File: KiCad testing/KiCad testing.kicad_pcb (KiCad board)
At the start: 2 copper layers, 101.6 x 127 mm, 37 parts, among them J1 USB_A, Q1 IRF540N, Q2 IRF540N, Q3 IRF540N, Q4 IRF540N, U1 IR2213, U4 IR2213

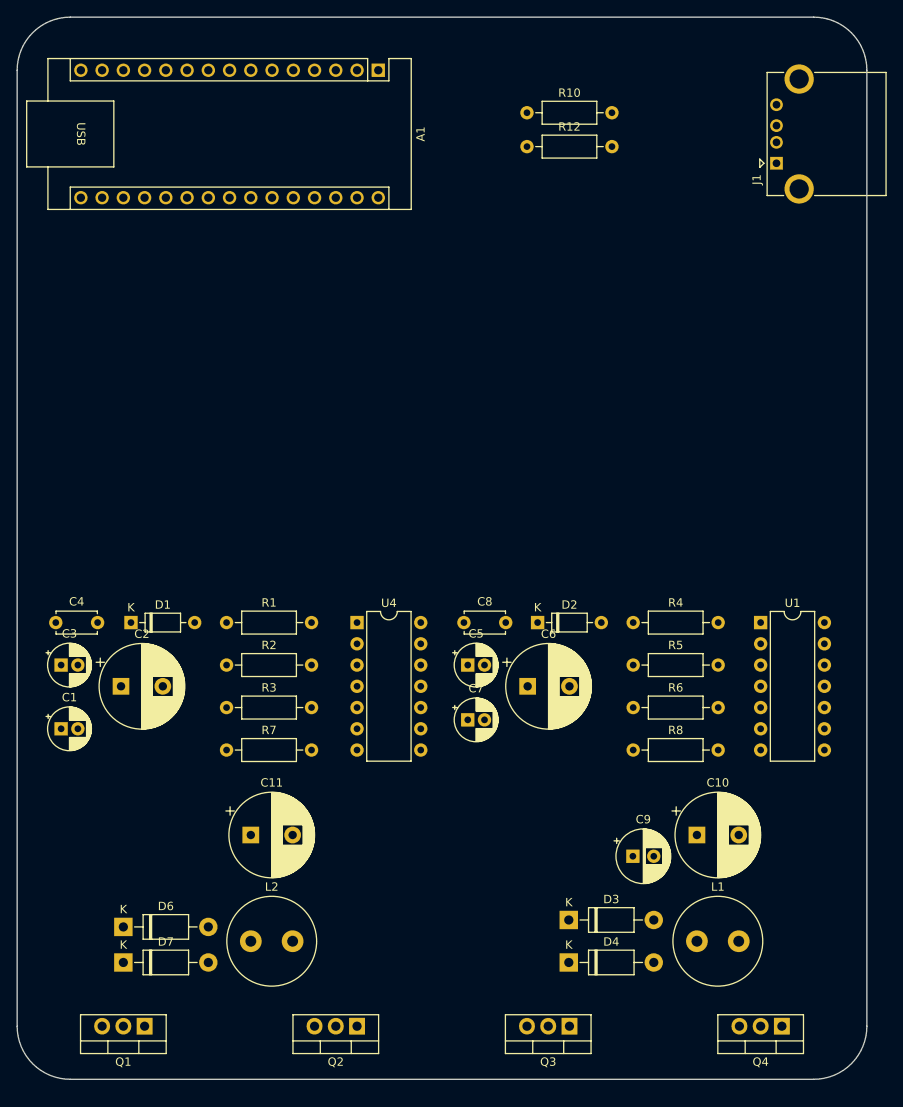
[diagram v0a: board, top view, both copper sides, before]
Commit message: update pcb
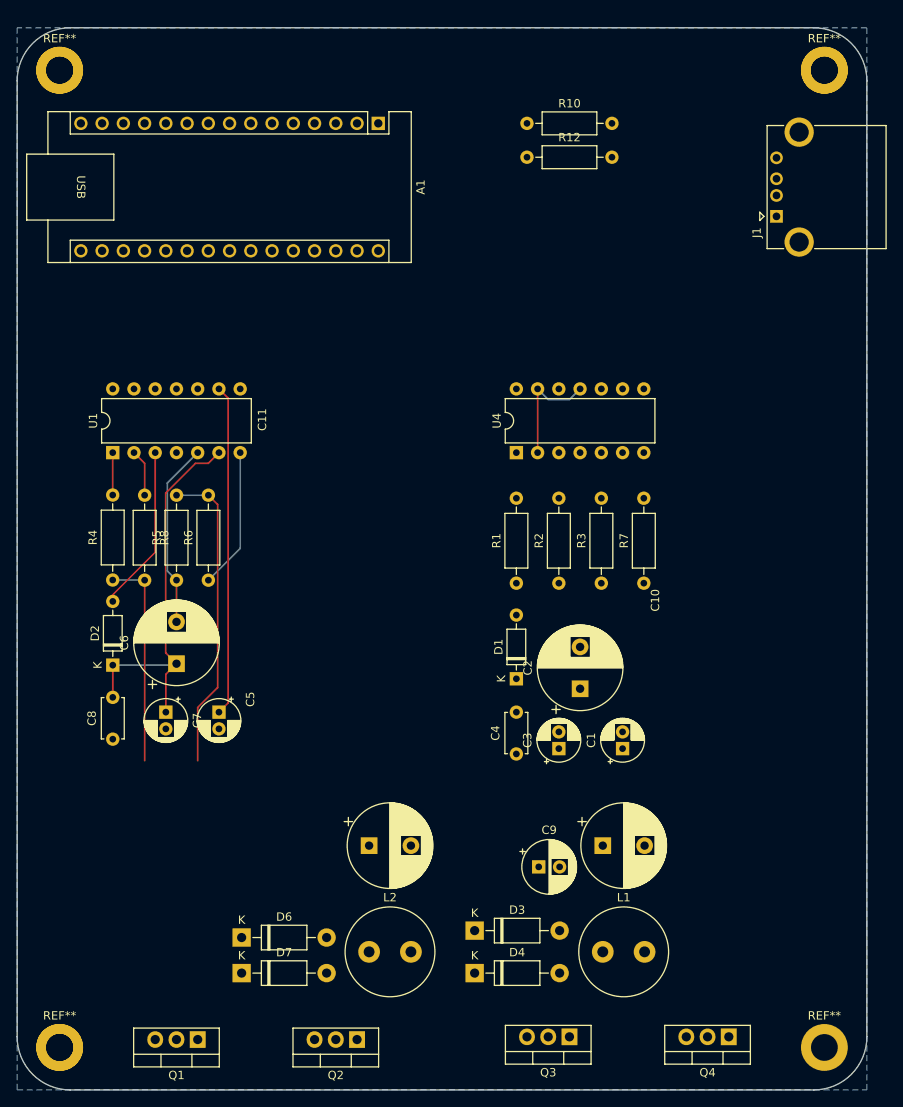
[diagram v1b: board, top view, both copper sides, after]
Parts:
- added ?: , , F.Cu at (121.9, 30.5)
- added ?: , , F.Cu at (30.5, 147.3)
- added ?: , , F.Cu at (30.5, 30.5)
- added REF**: MountingHole_3.2mm_M3_DIN965_Pad, MountingHole:MountingHole_3.2mm_M3_DIN965_Pad, F.Cu at (121.9, 30.5)
- added REF**: MountingHole_3.2mm_M3_DIN965_Pad, MountingHole:MountingHole_3.2mm_M3_DIN965_Pad, F.Cu at (30.5, 30.5)
- added REF**: MountingHole_3.2mm_M3_DIN965_Pad, MountingHole:MountingHole_3.2mm_M3_DIN965_Pad, F.Cu at (121.9, 147.3)
- added REF**: MountingHole_3.2mm_M3_DIN965_Pad, MountingHole:MountingHole_3.2mm_M3_DIN965_Pad, F.Cu at (30.5, 147.3)
- moved U1 80.1 mm to (36.8, 76.2), turned to 90 degrees
- moved C1 67.2 mm to (97.8, 111.6), turned to 90 degrees
- moved R8 65.9 mm to (40.6, 81.3), turned to -90 degrees
- moved R4 62.4 mm to (36.8, 91.4), turned to 90 degrees
- moved C3 60.3 mm to (90.2, 111.6), turned to 90 degrees
- moved C4 57.3 mm to (85.1, 112.2), turned to 90 degrees
- moved R5 55.5 mm to (44.5, 91.5), turned to 90 degrees
- moved C2 54.9 mm to (92.7, 104.4), turned to 90 degrees
- moved R7 53.7 mm to (100.3, 91.8), turned to 90 degrees
- moved R6 53.0 mm to (48.3, 91.5), turned to 90 degrees
- moved D2 51.0 mm to (36.8, 101.6), turned to 90 degrees
- moved R3 47.2 mm to (95.2, 91.8), turned to 90 degrees
- moved D1 46.6 mm to (85.1, 103.2), turned to 90 degrees
- moved C8 44.2 mm to (36.8, 110.5), turned to 90 degrees
- moved C6 42.1 mm to (44.5, 101.4), turned to 90 degrees
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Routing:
- net Net-(D2-K): track 0.00 -> 47.2 mm
- net 5V: track 0.00 -> 39.6 mm
- net Gate_High_1: track 0.00 -> 37.0 mm
- net Gate_Low_1: track 0.00 -> 25.4 mm
- net VS_1: track 0.00 -> 22.2 mm
- net 12V: track 0.00 -> 19.9 mm
- net GND: track 0.00 -> 19.4 mm
- net Net-(U1-HO): track 0.00 -> 16.8 mm
- net Net-(U1-LO): track 0.00 -> 5.07 mm
- added copper zone on B.Cu, net GND
